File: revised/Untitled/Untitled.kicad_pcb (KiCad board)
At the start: 2 copper layers, 168 x 134.2 mm, 42 parts, among them J1 Conn_01x02_Pin, J2 USB_C_Receptacle_USB2.0_16P, J3 ARM Cortex Debug, J4 Conn_Coaxial, J5 Screw_Terminal_01x02, J6 Screw_Terminal_01x02, J7 Screw_Terminal_01x02, Q1 Q_PMOS, Q2 NMOS, Q3 NMOS, U1 AP63205WU, U2 STM32F103C8Tx, U3 AMS1117-3.3, U6 SEEEDSTUDIOLORA

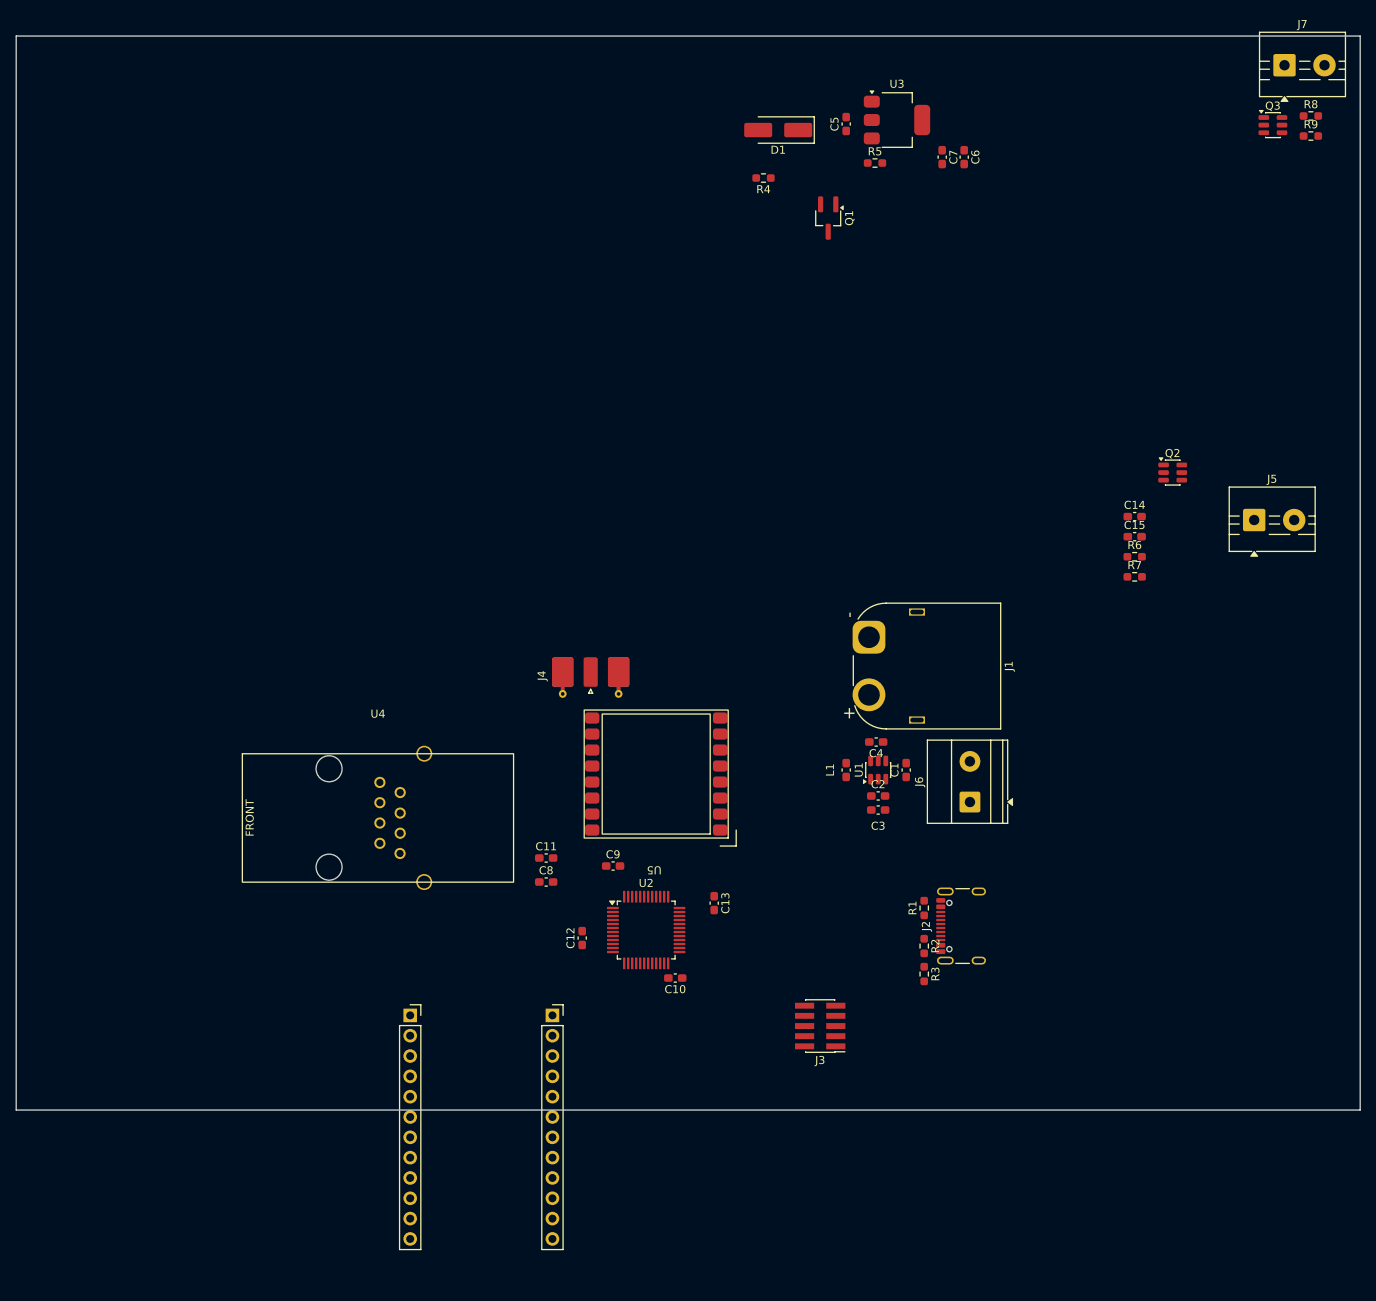
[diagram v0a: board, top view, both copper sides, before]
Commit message: layout revised
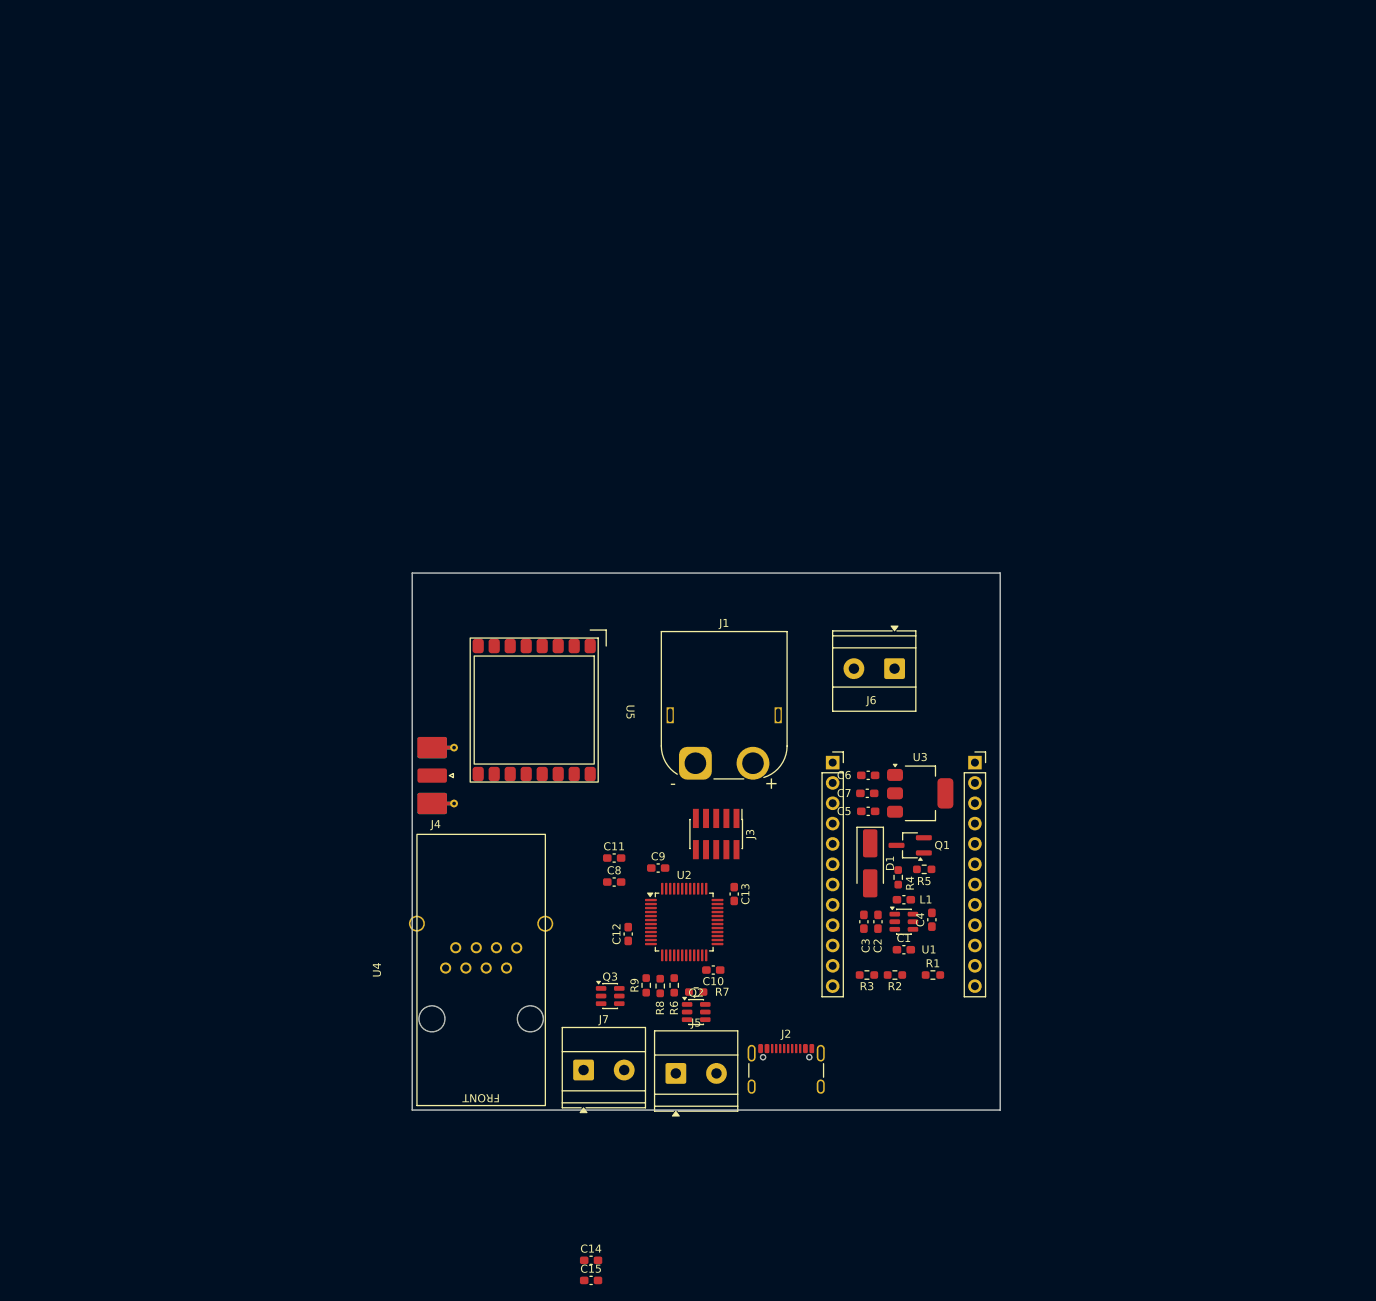
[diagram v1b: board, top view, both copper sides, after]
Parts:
- J5, J7: footprint TerminalBlock:TerminalBlock_MaiXu_MX126-5.0-02P_1x02_P5.00mm -> TerminalBlock_Phoenix:TerminalBlock_Phoenix_MKDS-1,5-2-5.08_1x02_P5.08mm_Horizontal
- moved J7 153.1 mm to (123.7, 144.8)
- moved Q3 136.8 mm to (127.0, 135.5)
- moved R8 135.8 mm to (133.2, 134.2), turned to 90 degrees
- moved R9 134.8 mm to (131.5, 134.2), turned to 90 degrees
- moved C15 115.2 mm to (124.6, 171.0)
- moved C14 115.2 mm to (124.6, 168.5)
- moved J5 100.1 mm to (135.2, 145.2)
- moved D1 92.4 mm to (159.5, 118.9), turned to -90 degrees
- moved Q2 90.0 mm to (137.8, 137.5)
- moved R4 89.0 mm to (163.0, 120.7), turned to -90 degrees
- moved R5 88.5 mm to (166.2, 119.7)
- moved C5 86.0 mm to (159.2, 112.4), turned to 180 degrees
- moved U3 84.2 mm to (165.8, 110.2)
- moved C7 80.1 mm to (159.1, 110.2), turned to 180 degrees
- moved Q1 79.1 mm to (164.5, 116.7), turned to 180 degrees
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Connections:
- Q2 pad 1: Net-(J5-Pin_1) -> Net-(J5-Pin_2)
- Q2 pad 3: Net-(J5-Pin_2) -> Net-(J5-Pin_1)
- Q3 pad 1: Net-(J7-Pin_1) -> Net-(J7-Pin_2)
- Q3 pad 3: Net-(J7-Pin_2) -> Net-(J7-Pin_1)
- U2 pad 26: SWDIO -> RADIO_SCK
- U2 pad 27: SWCLK -> RADIO_MISO
- U2 pad 28: unconnected-(U2-PB15-Pad28) -> RADIO_MOSI
- U2 pad 34: RADIO_SCK -> SWDIO
- U2 pad 37: RADIO_MISO -> SWCLK
- U2 pad 38: RADIO_MOSI -> unconnected-(U2-PA15-Pad38)
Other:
- board size 168 x 134.2 mm -> 73.5 x 67.1 mm

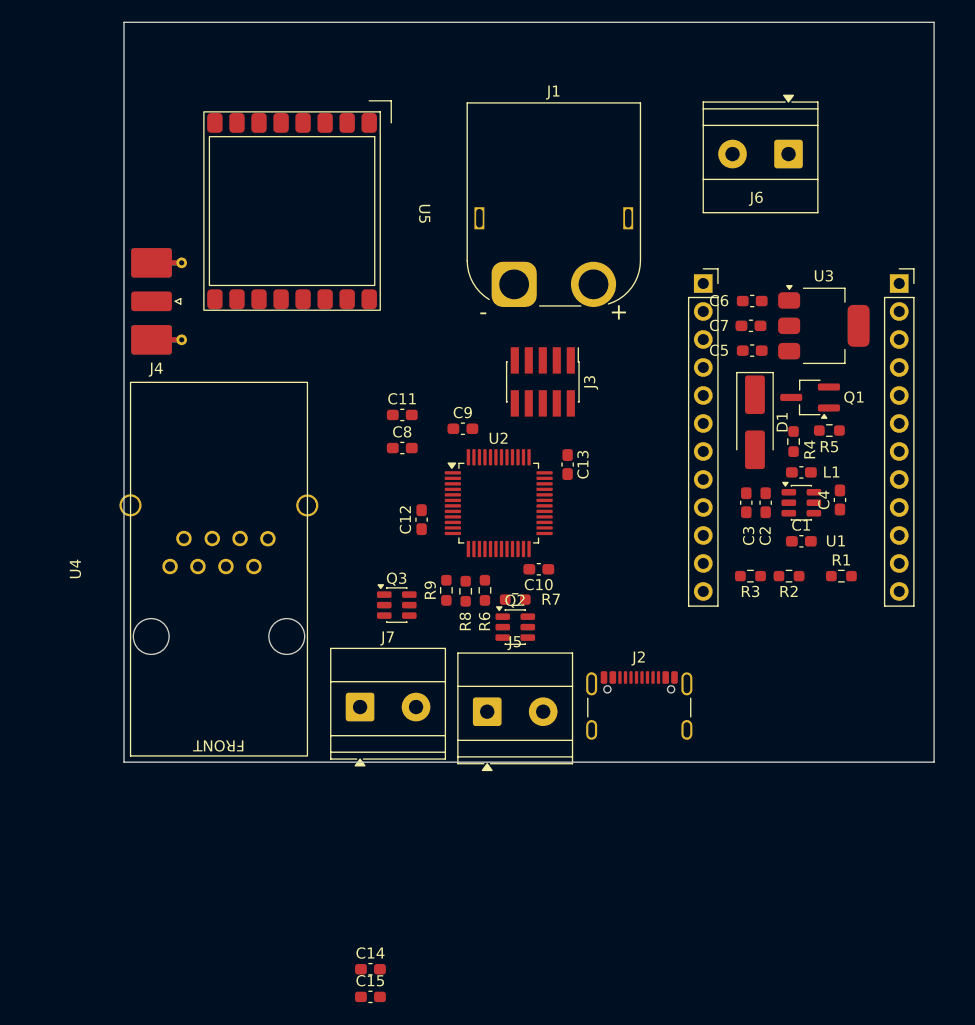
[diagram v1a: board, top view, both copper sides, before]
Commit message: signal routing start
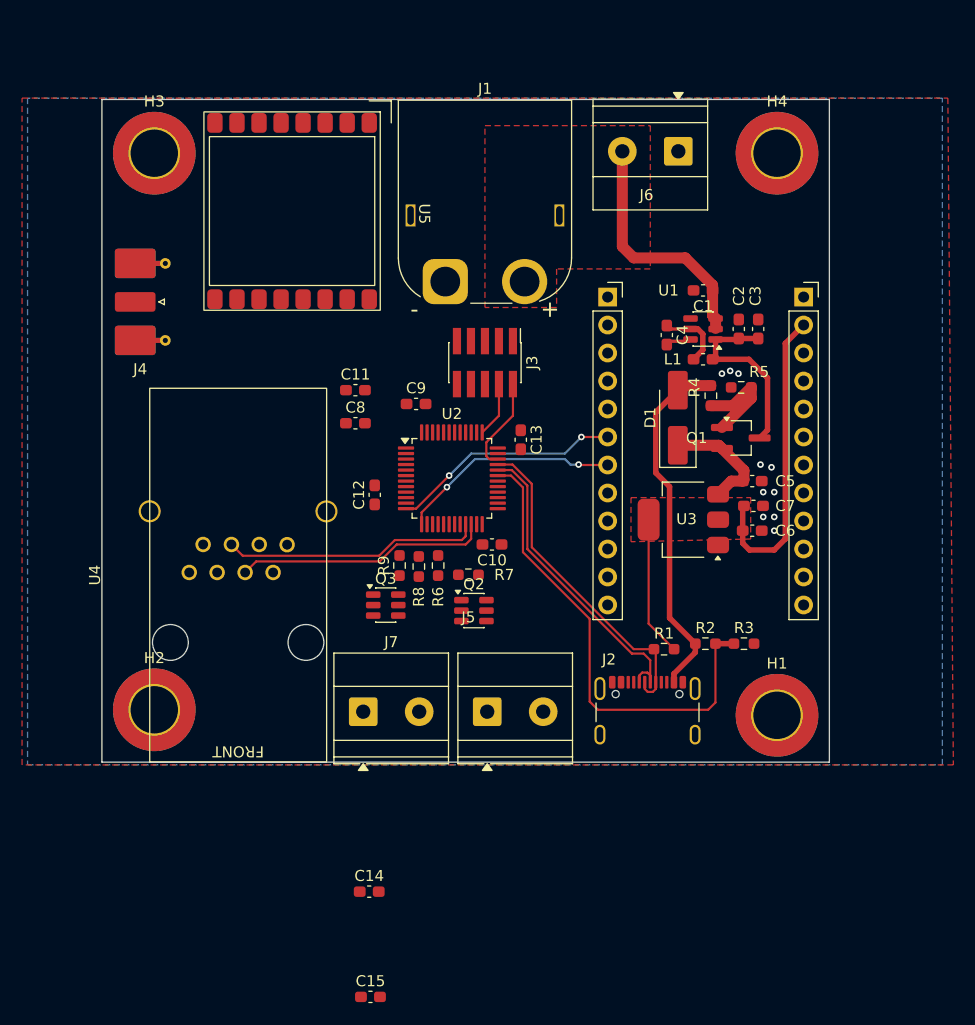
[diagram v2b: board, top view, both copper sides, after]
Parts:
- added H1: MountingHole_Pad, MountingHole:MountingHole_4.3mm_M4_DIN965_Pad_TopBottom, F.Cu at (161.5, 145.5)
- added H2: MountingHole_Pad, MountingHole:MountingHole_4.3mm_M4_DIN965_Pad_TopBottom, F.Cu at (105.0, 145.0)
- added H3: MountingHole_Pad, MountingHole:MountingHole_4.3mm_M4_DIN965_Pad_TopBottom, F.Cu at (105.0, 94.5)
- added H4: MountingHole_Pad, MountingHole:MountingHole_4.3mm_M4_DIN965_Pad_TopBottom, F.Cu at (161.5, 94.5)
- moved C1 24.4 mm to (154.8, 107.0), turned to 180 degrees
- moved U3 21.7 mm to (153.0, 127.8), turned to 180 degrees
- moved C4 21.7 mm to (151.5, 111.0), turned to -90 degrees
- moved C6 20.8 mm to (159.2, 128.8), turned to 0 degrees
- moved U1 18.1 mm to (154.8, 110.5), turned to 180 degrees
- moved R1 17.4 mm to (151.2, 139.5)
- moved C7 16.3 mm to (159.4, 126.5), turned to 0 degrees
- moved C2 16.0 mm to (158.0, 110.5), turned to 90 degrees
- moved C3 15.8 mm to (159.8, 110.5), turned to 90 degrees
- moved L1 13.6 mm to (154.8, 113.2), turned to 0 degrees
- moved C5 11.8 mm to (159.2, 124.2), turned to 0 degrees
- moved J6 10.0 mm to (152.5, 94.3)
- moved R2 9.75 mm to (155.0, 139.0), turned to 0 degrees
- moved R5 8.91 mm to (158.2, 115.8), turned to 180 degrees
- moved U6 8.76 mm to (146.1, 107.5)
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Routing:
- net USB_DETECT: track 0.00 -> 43.7 mm
- net +3.3V: track 0.00 -> 40.4 mm
- net USB5V: track 0.00 -> 32.8 mm
- net USB_DP: track 0.00 -> 30.0 mm
- net USB_DM: track 0.00 -> 28.8 mm
- net STM_TX_ETH_RX: track 0.00 -> 23.5 mm
- net STM_RX_ETH_TX: track 0.00 -> 23.1 mm
- net +8V: track 0.00 -> 22.3 mm
- net STM_TX_LORA_RX: track 0.00 -> 21.0 mm, vias 0 -> 2
- net STM_RX_LORA_TX: track 0.00 -> 20.2 mm, vias 0 -> 2
- net +5V: track 0.00 -> 17.2 mm
- net Net-(D1-K): track 0.00 -> 10.7 mm
- net Net-(Q1-G): track 0.00 -> 9.09 mm
- net SWDIO: track 0.00 -> 8.68 mm
- net Net-(U1-SW): track 0.00 -> 6.99 mm
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- added copper zone on F.Cu, net +3.3V
- added copper zone on F.Cu, net +8V
- added copper zone on B.Cu, net GND
- added copper zone on F.Cu, net GND
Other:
- board size 73.5 x 67.1 mm -> 66 x 60.1 mm
